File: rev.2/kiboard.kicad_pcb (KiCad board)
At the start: 2 copper layers, 127.3 x 101 mm, 38 parts

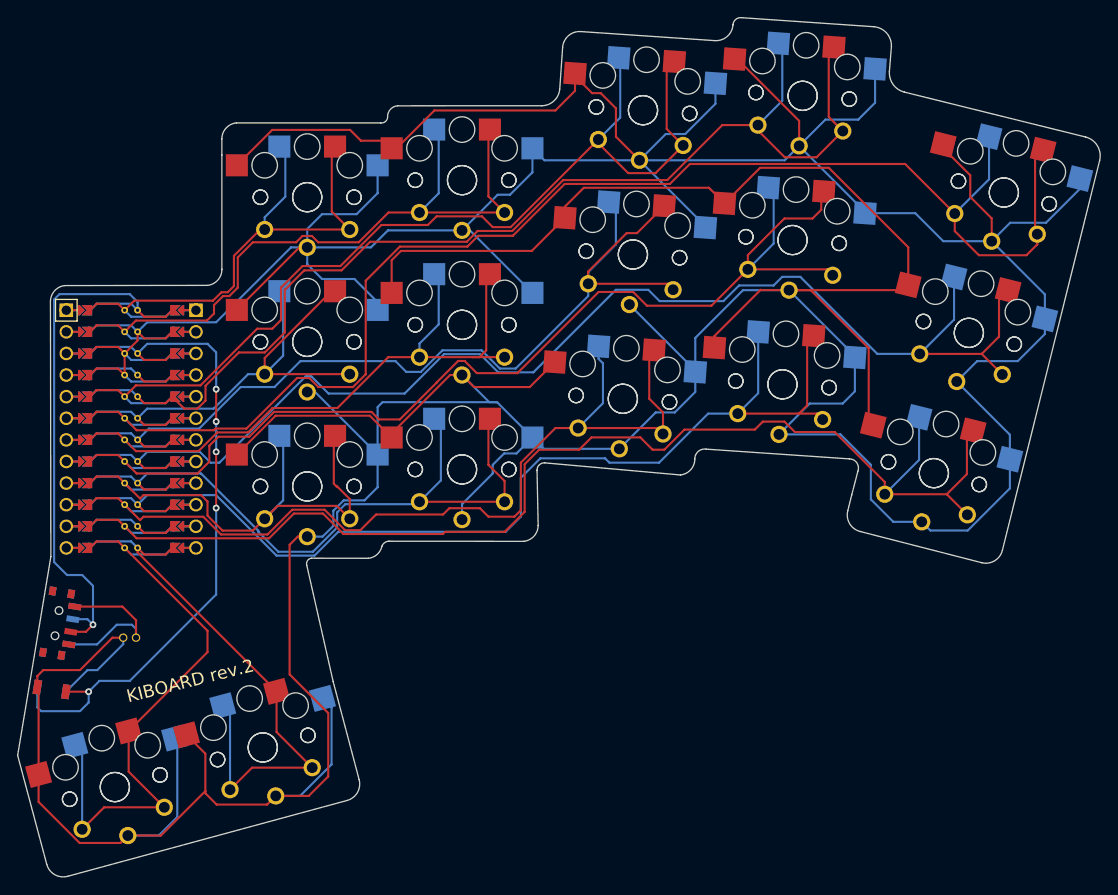
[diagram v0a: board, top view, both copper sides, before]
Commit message: feat!: rev3 WIP
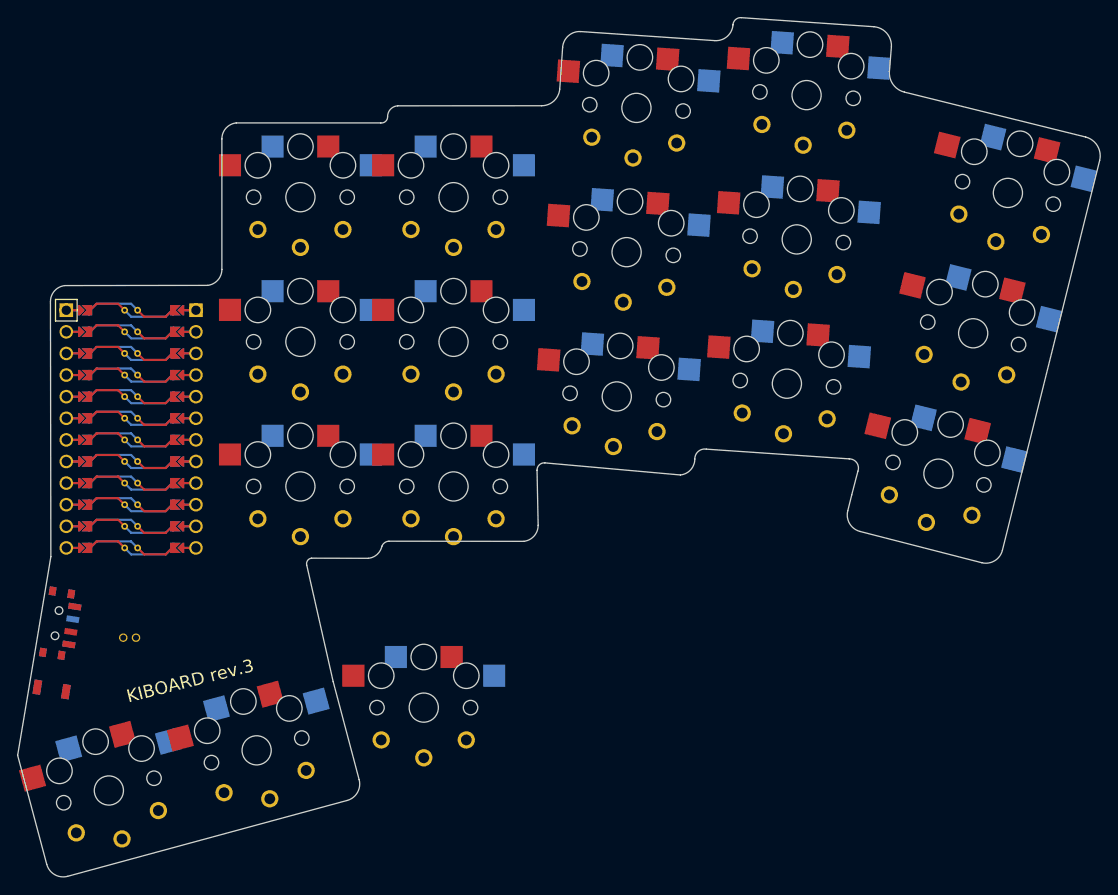
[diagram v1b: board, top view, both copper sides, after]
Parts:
- removed S1, S10, S11, S12, S13, S14, S15, S16, S17, S18, S19, S2, S20, S21, S22, S23, S24, S25, S26, S27, S28, S29, S3, S30, S31, S32, S33, S34, S4, S5, S6, S7, S8, S9: , PG1350
- added SW: , keyswitches:SW_Kailh_Reversible, F.Cu at (75.5, -46.0)
- added SW: , keyswitches:SW_Kailh_Reversible, F.Cu at (10.9, 31.0)
- added SW: , keyswitches:SW_Kailh_Reversible, F.Cu at (34.0, -34.0)
- added SW: , keyswitches:SW_Kailh_Reversible, F.Cu at (54.3, -27.5)
- added SW: , keyswitches:SW_Kailh_Reversible, F.Cu at (74.3, -29.0)
- added SW: , keyswitches:SW_Kailh_Reversible, F.Cu at (91.0, -1.50)
- added SW: , keyswitches:SW_Kailh_Reversible, F.Cu at (55.5, -44.5)
- added SW: , keyswitches:SW_Kailh_Reversible, F.Cu at (34.0, -17.0)
- added SW: , keyswitches:SW_Kailh_Reversible, F.Cu at (73.2, -12.1)
- added SW: , keyswitches:SW_Kailh_Reversible, F.Cu at (16.0, 0.00)
- added SW: , keyswitches:SW_Kailh_Reversible, F.Cu at (16.0, -17.0)
- added SW: , keyswitches:SW_Kailh_Reversible, F.Cu at (34.0, 0.00)
- added SW: , keyswitches:SW_Kailh_Reversible, F.Cu at (-6.52, 35.7)
- added SW: , keyswitches:SW_Kailh_Reversible, F.Cu at (95.1, -18.0)
- added SW: , keyswitches:SW_Kailh_Reversible, F.Cu at (30.5, 26.0)
- added SW: , keyswitches:SW_Kailh_Reversible, F.Cu at (99.2, -34.5)
- added SW: , keyswitches:SW_Kailh_Reversible, F.Cu at (16.0, -34.0)
- added SW: , keyswitches:SW_Kailh_Reversible, F.Cu at (53.2, -10.6)
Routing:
- net GND: track 867.7 -> 0.00 mm
- net Switch05: track 156.6 -> 0.00 mm
- net Switch10: track 140.5 -> 0.00 mm
- net Switch15: track 136.3 -> 0.00 mm
- net Switch09: track 124.2 -> 0.00 mm
- net Switch04: track 120.7 -> 0.00 mm
- net Switch14: track 113.2 -> 0.00 mm
- net Switch03: track 105.1 -> 0.00 mm
- net Switch08: track 99.4 -> 0.00 mm
- net Switch13: track 98.4 -> 0.00 mm
- net Switch02: track 73.9 -> 0.00 mm
- net Switch07: track 72.8 -> 0.00 mm
- net Switch12: track 72.7 -> 0.00 mm
- net RST: track 71.3 -> 0.00 mm, vias 5 -> 0
- net Switch16: track 61.1 -> 0.00 mm
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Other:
- board text added: "KIBOARD rev.3"
- board text removed: "KIBOARD rev.2"
